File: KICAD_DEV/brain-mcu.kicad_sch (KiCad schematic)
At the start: 13 parts, among them SW1 SW_Push, U1 STM32H743VITx

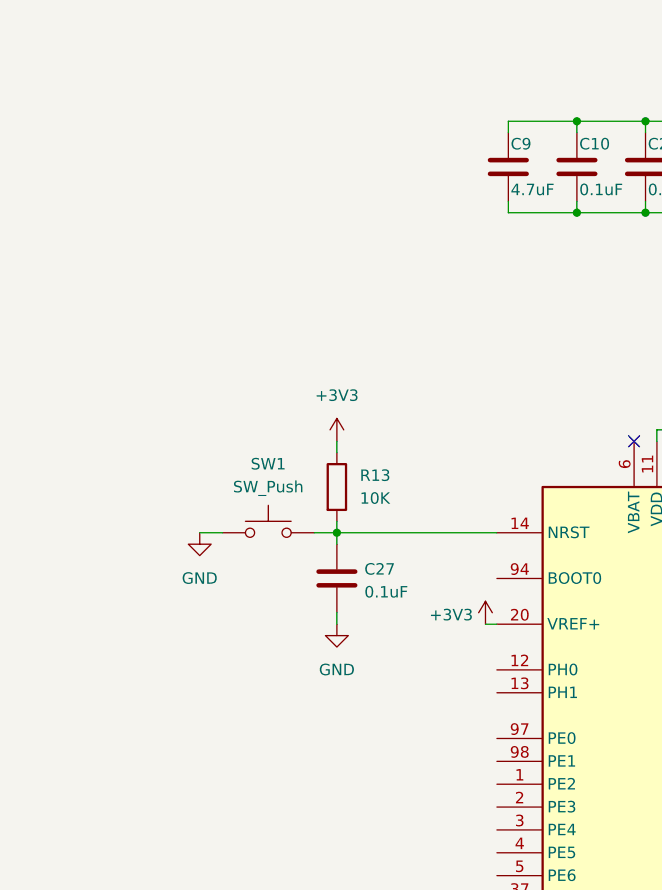
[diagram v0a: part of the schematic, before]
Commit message: more cleaning up and adding boot
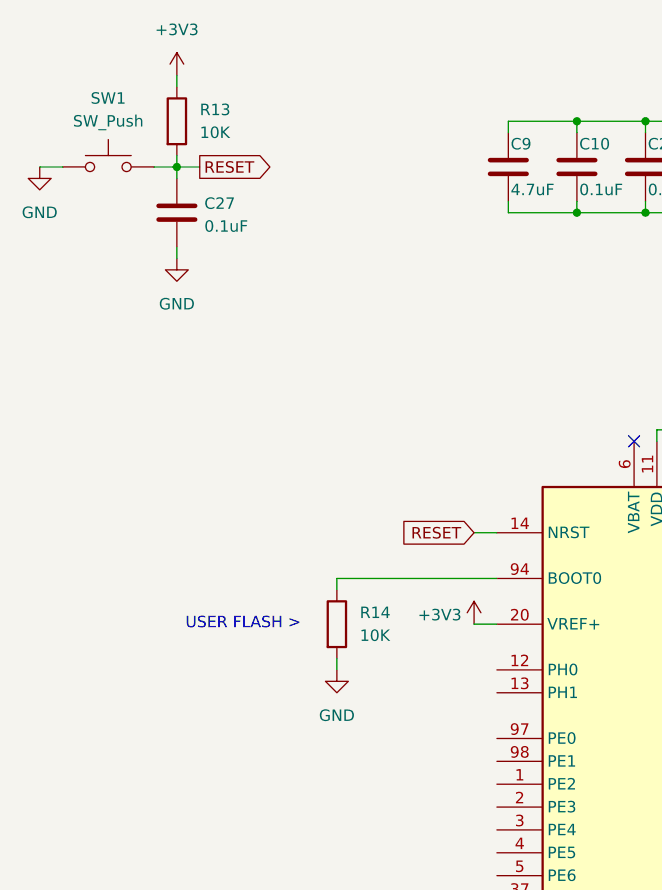
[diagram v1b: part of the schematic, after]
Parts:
- added R14: 10K, symbol Device:R
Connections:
- net GND: now also R14.2
- net RESET: now reaches C27.1, R13.2, SW1.2, U1.14 (NRST)
- net at U1.94 (BOOT0): now also R14.1
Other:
- note added: "USER FLASH >"
- moved on the sheet: C27, R13, SW1
